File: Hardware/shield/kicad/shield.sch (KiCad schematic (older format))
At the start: 26 parts

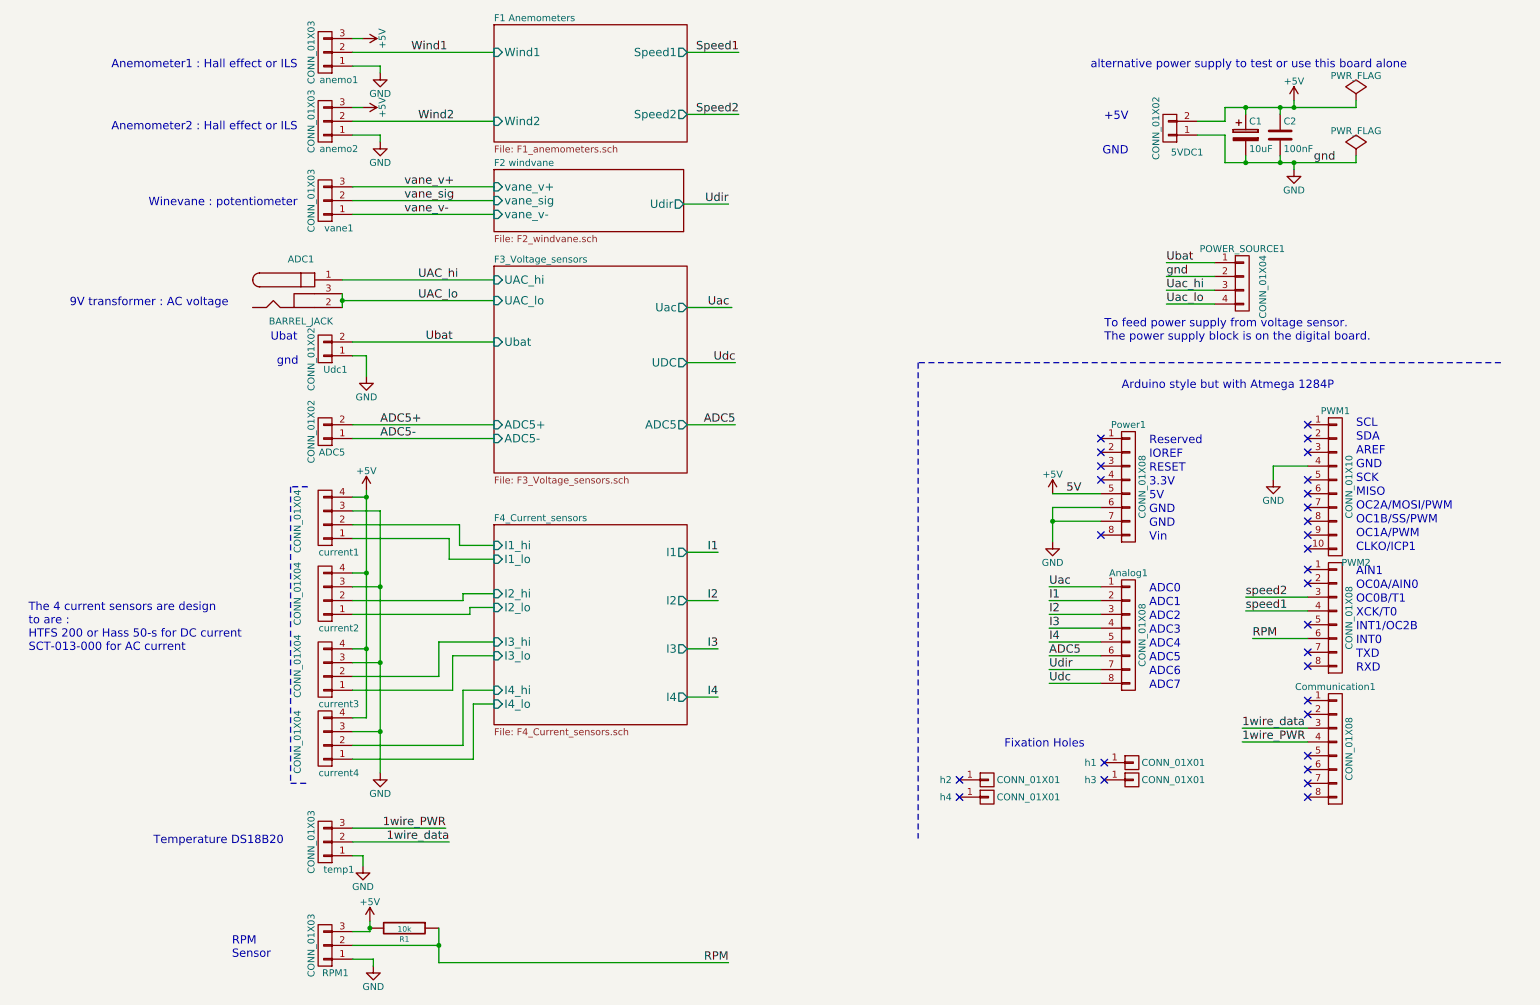
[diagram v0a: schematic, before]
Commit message: move to digital 1.1.1
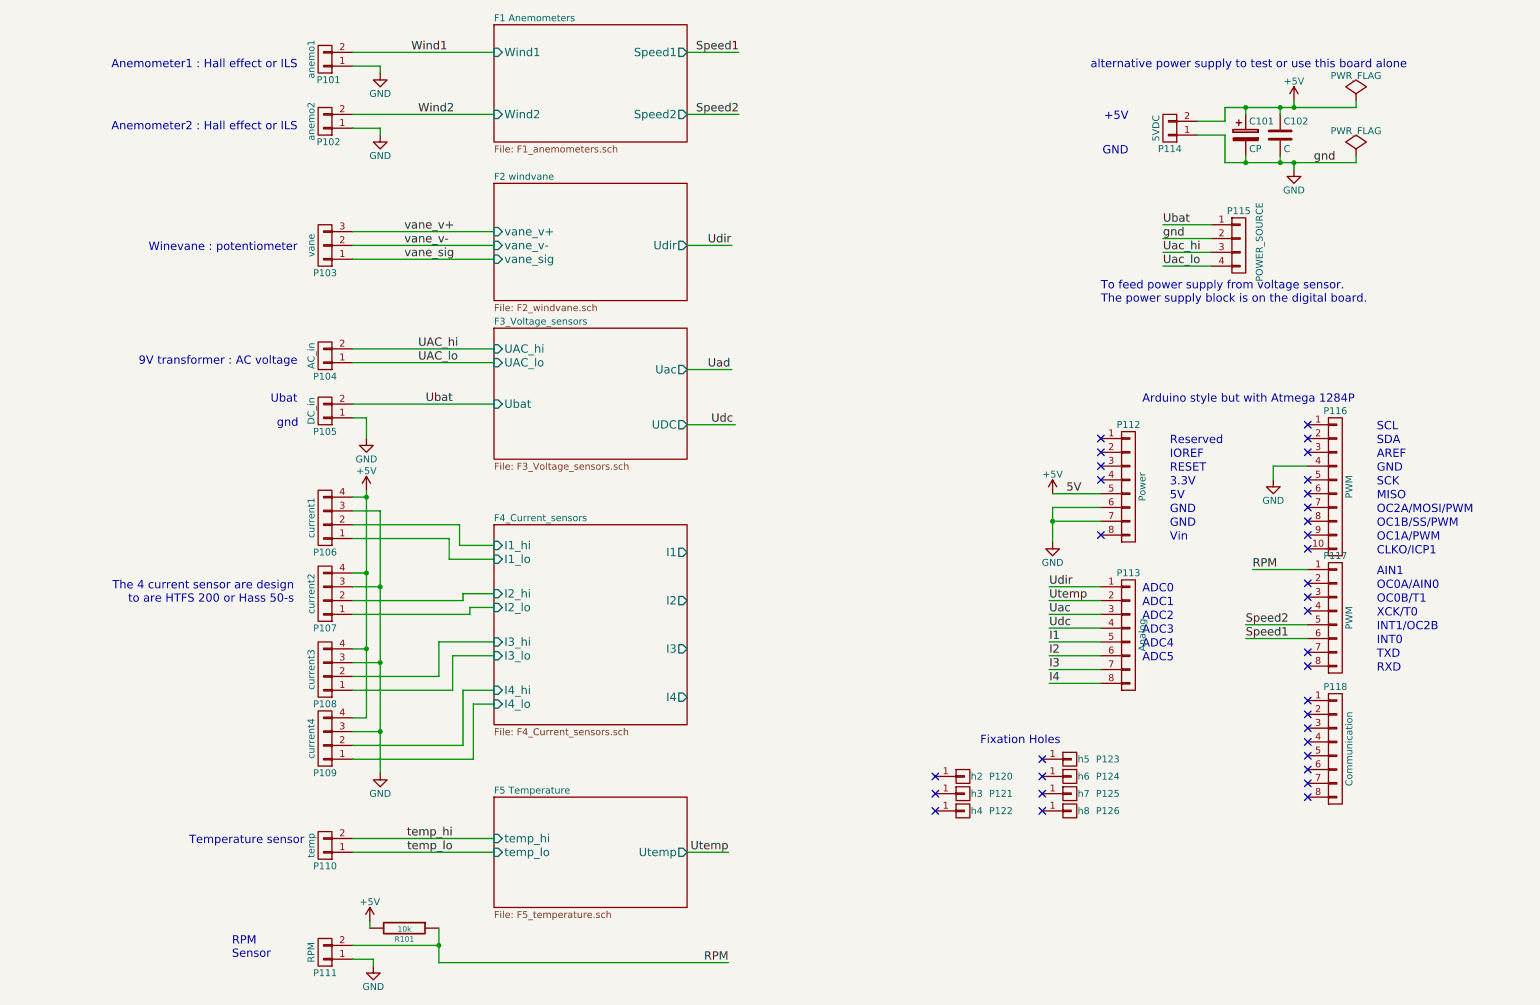
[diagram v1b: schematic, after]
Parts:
- removed 5VDC1: CONN_01X02, Socket_Strips:Socket_Strip_Straight_1x02, symbol CONN_01X02
- removed ADC1: BARREL_JACK, Connect:BARREL_JACK, symbol BARREL_JACK
- removed ADC5, Udc1: CONN_01X02, w_conn_screw:mstba_2,5%2f2-g-5,08, symbol CONN_01X02
- removed Analog1, Communication1, PWM2, Power1: CONN_01X08, Socket_Arduino_Mega:Socket_Strip_Arduino_1x08, symbol CONN_01X08
- removed POWER_SOURCE1: CONN_01X04, Socket_Strips:Socket_Strip_Straight_1x04, symbol CONN_01X04
- removed PWM1: CONN_01X10, Socket_Arduino_Mega:Socket_Strip_Arduino_1x10, symbol CONN_01X10
- removed RPM1, anemo1, anemo2, temp1, vane1: CONN_01X03, w_conn_screw:mstba_2,5%2f3-g-5,08, symbol CONN_01X03
- removed current1, current2, current3, current4: CONN_01X04, w_conn_screw:mstba_2,5%2f4-g-5,08, symbol CONN_01X04
- removed h1, h2, h3, h4: CONN_01X01, Socket_Arduino_Mega:Arduino_1pin, symbol CONN_01X01
- added P101: anemo1, Terminal_Blocks:TerminalBlock_Pheonix_MKDS1.5-2pol, symbol CONN_01X02
- added P102: anemo2, Terminal_Blocks:TerminalBlock_Pheonix_MKDS1.5-2pol, symbol CONN_01X02
- added P103: vane, Terminal_Blocks:TerminalBlock_Pheonix_MKDS1.5-3pol, symbol CONN_01X03
- added P104: AC_in, Terminal_Blocks:TerminalBlock_Pheonix_MKDS1.5-2pol, symbol CONN_01X02
- added P105: DC_in, Terminal_Blocks:TerminalBlock_Pheonix_MKDS1.5-2pol, symbol CONN_01X02
- added P106: current1, Terminal_Blocks:TerminalBlock_Pheonix_MKDS1.5-4pol, symbol CONN_01X04
- added P107: current2, Terminal_Blocks:TerminalBlock_Pheonix_MKDS1.5-4pol, symbol CONN_01X04
- added P108: current3, Terminal_Blocks:TerminalBlock_Pheonix_MKDS1.5-4pol, symbol CONN_01X04
- added P109: current4, Terminal_Blocks:TerminalBlock_Pheonix_MKDS1.5-4pol, symbol CONN_01X04
- added P110: temp, Terminal_Blocks:TerminalBlock_Pheonix_MKDS1.5-2pol, symbol CONN_01X02
- added P111: RPM, Terminal_Blocks:TerminalBlock_Pheonix_MKDS1.5-2pol, symbol CONN_01X02
- added P112: Power, Socket_Arduino_Mega:Socket_Strip_Arduino_1x08, symbol CONN_01X08
- added P113: Analog, Socket_Arduino_Mega:Socket_Strip_Arduino_1x08, symbol CONN_01X08
- added P114: 5VDC, Socket_Strips:Socket_Strip_Straight_1x02, symbol CONN_01X02
- added P115: POWER_SOURCE, Socket_Strips:Socket_Strip_Straight_1x04, symbol CONN_01X04
- added P116: PWM, Socket_Arduino_Mega:Socket_Strip_Arduino_1x10, symbol CONN_01X10
- added P117: PWM, Socket_Arduino_Mega:Socket_Strip_Arduino_1x08, symbol CONN_01X08
- added P118: Communication, Socket_Arduino_Mega:Socket_Strip_Arduino_1x08, symbol CONN_01X08
- added P120: h2, Socket_Arduino_Mega:Arduino_1pin, symbol CONN_01X01
- added P121: h3, Socket_Arduino_Mega:Arduino_1pin, symbol CONN_01X01
- added P122: h4, Socket_Arduino_Mega:Arduino_1pin, symbol CONN_01X01
- added P123: h5, Socket_Arduino_Mega:Arduino_1pin, symbol CONN_01X01
- added P124: h6, Socket_Arduino_Mega:Arduino_1pin, symbol CONN_01X01
- added P125: h7, Socket_Arduino_Mega:Arduino_1pin, symbol CONN_01X01
- added P126: h8, Socket_Arduino_Mega:Arduino_1pin, symbol CONN_01X01
- C101: renamed from C1; value 10uF -> CP
- C102: renamed from C2; value 100nF -> C; footprint Capacitors_ThroughHole:C_Rect_L7_W2.5_P5 -> Capacitors_ThroughHole:C_Radial_D5_L6_P2.5
- R101: renamed from R1; footprint Discret:R3-LARGE_PADS -> Discret:R4
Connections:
- net +5V: now also P106.4 (P4), P107.4 (P4), P108.4 (P4), P109.4 (P4), P112.5 (P5), P114.2 (P2)
- net F4_Current_sensors/I1_hi: now also P106.2 (P2)
- net F4_Current_sensors/I1_lo: now also P106.1 (P1)
- net F4_Current_sensors/I2_hi: now also P107.2 (P2)
- net F4_Current_sensors/I2_lo: now also P107.1 (P1)
- net F4_Current_sensors/I3_hi: now also P108.2 (P2)
- net F4_Current_sensors/I3_lo: now also P108.1 (P1)
- net F4_Current_sensors/I4_hi: now also P109.2 (P2)
- net F4_Current_sensors/I4_lo: now also P109.1 (P1)
- net GND: now also P101.1 (P1), P102.1 (P1), P105.1 (P1), P106.3 (P3), P107.3 (P3), P108.3 (P3), P109.3 (P3), P111.1 (P1), P112.6 (P6), P112.7 (P7), P114.1 (P1), P115.2 (P2), P116.4 (P4)
- net I1: now also P113.5 (P5)
- net I2: now also P113.6 (P6)
- net I3: now also P113.7 (P7)
- net I4: now also P113.8 (P8)
- net RPM: now also P111.2 (P2), P117.1 (P1)
- net Speed1: now also P117.6 (P6)
- net Speed2: now also P117.5 (P5)
- net UAC_hi: now also P104.2 (P2)
- net UAC_lo: now also P104.1 (P1)
- net Uac: now also P113.3 (P3)
- net Uac_hi: now also P115.3 (P3)
- net Uac_lo: now also P115.4 (P4)
- net Ubat: now also P105.2 (P2), P115.1 (P1)
- net Udc: now also P113.4 (P4)
- net Udir: now also P113.1 (P1)
- net Wind1: now also P101.2 (P2)
- net Wind2: now also P102.2 (P2)
- net vane_sig: now also P103.1 (P1)
- net vane_v+: now also P103.3 (P3)
- net vane_v-: now also P103.2 (P2)
- new net Utemp: P113.2 (P2)
- new net temp_hi: P110.2 (P2)
- new net temp_lo: P110.1 (P1)
- no-connect marks 29 -> 34
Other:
- note added: "Temperature sensor"
- note added: "The 4 current sensor are design \nto are HTFS 200 or Hass 50-s"
- note removed: "ADC6"
- note removed: "ADC7"
- note removed: "Temperature DS18B20"
- note removed: "The 4 current sensors are design \nto are :\nHTFS 200 or Hass 50-s for DC current\nSCT-013-000 for AC current"
